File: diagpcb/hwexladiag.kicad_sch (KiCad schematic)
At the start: 0 parts

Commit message: Add HC05 symbol & footprint.
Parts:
- added J1: PINHEADER, Connector_PinHeader_2.54mm:PinHeader_1x06_P2.54mm_Vertical_SMD_Pin1Left, symbol Connector_Generic:Conn_01x06
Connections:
- new net +5V: J1.4 (Pin_4)
- new net GND: J1.6 (Pin_6)
- new net wexlaRxD: J1.3 (Pin_3)
- new net wexlaTxD: J1.2 (Pin_2)
- no-connect marks 0 -> 2
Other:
- company: (none) -> Model Railroader Club Brno I – KMŽ Brno I – https://kmz-brno.cz/
- title: (none) -> hWexla Wireless Diagnostic Adapter
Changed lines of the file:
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@@
 (kicad_sch (version 20230121) (generator eeschema)
   (paper "A5")
+  (title_block
+    (title "hWexla Wireless Diagnostic Adapter")
+    (date "2023-12-16")
+    (rev "1.0")
+    (company "Model Railroader Club Brno I – KMŽ Brno I – https://kmz-brno.cz/")
+    (comment 1 "Jan Horáček")
+    (comment 2 "https://github.com/kmzbrnoI/hwexla")
+    (comment 3 "https://creativecommons.org/licenses/by-sa/4.0/")
+    (comment 4 "Released under the Creative Commons Attribution-ShareAlike 4.0 License")
+  )
+  (no_connect (at 124.46 55.245))
+  (no_connect (at 124.46 65.405))
+  (wire (pts (xy 124.46 57.785) (xy 104.14 57.785))
+    (stroke (width 0) (type default))
+  )
+  (wire (pts (xy 111.76 62.865) (xy 124.46 62.865))
+    (stroke (width 0) (type default))
+  )
+  (wire (pts (xy 115.57 71.12) (xy 115.57 67.945))
+    (stroke (width 0) (type default))
+  )
+  (wire (pts (xy 111.76 52.07) (xy 111.76 62.865))
+    (stroke (width 0) (type default))
+  )
+  (wire (pts (xy 104.14 60.325) (xy 124.46 60.325))
+    (stroke (width 0) (type default))
+  )
+  (wire (pts (xy 115.57 67.945) (xy 124.46 67.945))
+    (stroke (width 0) (type default))
+  )
+  (label "wexlaRxD" (at 122.555 60.325 180) (fields_autoplaced)
+    (effects (font (size 1.27 1.27)) (justify right bottom))
+  )
+  (label "wexlaTxD" (at 122.555 57.785 180) (fields_autoplaced)
+    (effects (font (size 1.27 1.27)) (justify right bottom))
+  )
+  (symbol (lib_id "power:GND") (at 115.57 71.12 0) (unit 1)
+    (in_bom yes) (on_board yes) (dnp no) (fields_autoplaced)
+    (property "Reference" "#PWR01" (at 115.57 77.47 0)
+      (effects (font (size 1.27 1.27)) hide)
+    )
+    (property "Value" "GND" (at 115.57 75.2531 0)
+      (effects (font (size 1.27 1.27)))
+    )
+    (property "Footprint" "" (at 115.57 71.12 0)
+      (effects (font (size 1.27 1.27)) hide)
+    )
+    (property "Datasheet" "" (at 115.57 71.12 0)
+      (effects (font (size 1.27 1.27)) hide)
+    )
+    (pin "1")
+    (instances
+      (project "hwexladiag"
+        (path "/41af901d-6d9d-4dc3-adca-d33b9d619d2e"
+          (reference "#PWR01") (unit 1)
+        )
+      )
+    )
+  )
+  (symbol (lib_id "Connector_Generic:Conn_01x06") (at 129.54 60.325 0) (unit 1)
+    (in_bom yes) (on_board yes) (dnp no) (fields_autoplaced)
+    (property "Reference" "J1" (at 131.572 60.3829 0)
+      (effects (font (size 1.27 1.27)) (justify left))
+    )
+    (property "Value" "PINHEADER" (at 131.572 62.8071 0)
+      (effects (font (size 1.27 1.27)) (justify left))
+    )
+    (property "Footprint" "Connector_PinHeader_2.54mm:PinHeader_1x06_P2.54mm_Vertical_SMD_Pin1Left" (at 129.54 60.325 0)
+      (effects (font (size 1.27 1.27)) hide)
+    )
+    (property "Datasheet" "~" (at 129.54 60.325 0)
+      (effects (font (size 1.27 1.27)) hide)
+    )
+    (pin "1")
+    (pin "2")
+    (pin "3")
+    (pin "4")
+    (pin "5")
+    (pin "6")
+    (instances
+      (project "hwexladiag"
+        (path "/41af901d-6d9d-4dc3-adca-d33b9d619d2e"
+          (reference "J1") (unit 1)
+        )
+      )
+    )
+  )
+  (symbol (lib_id "power:+5V") (at 111.76 52.07 0) (unit 1)
+    (in_bom yes) (on_board yes) (dnp no) (fields_autoplaced)
+    (property "Reference" "#PWR02" (at 111.76 55.88 0)
+      (effects (font (size 1.27 1.27)) hide)
+    )
+    (property "Value" "+5V" (at 111.76 47.9369 0)
+      (effects (font (size 1.27 1.27)))
+    )
+    (property "Footprint" "" (at 111.76 52.07 0)
+      (effects (font (size 1.27 1.27)) hide)
+    )
+    (property "Datasheet" "" (at 111.76 52.07 0)
+      (effects (font (size 1.27 1.27)) hide)
+    )
+    (pin "1")
+    (instances
+      (project "hwexladiag"
+        (path "/41af901d-6d9d-4dc3-adca-d33b9d619d2e"
+          (reference "#PWR02") (unit 1)
+        )
+      )
+    )
+  )
   (sheet_instances
     (path "/" (page "1"))

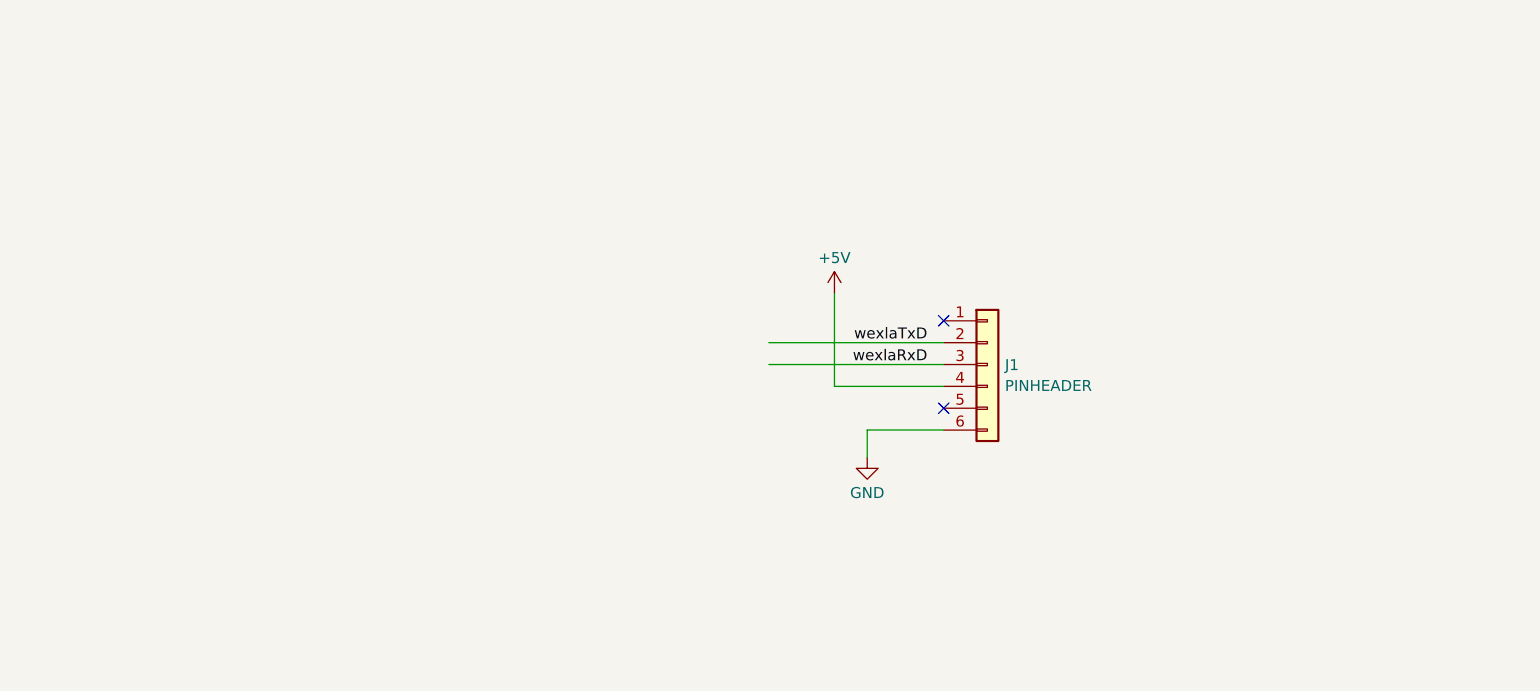
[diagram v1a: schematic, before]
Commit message: Finish diagPCB.
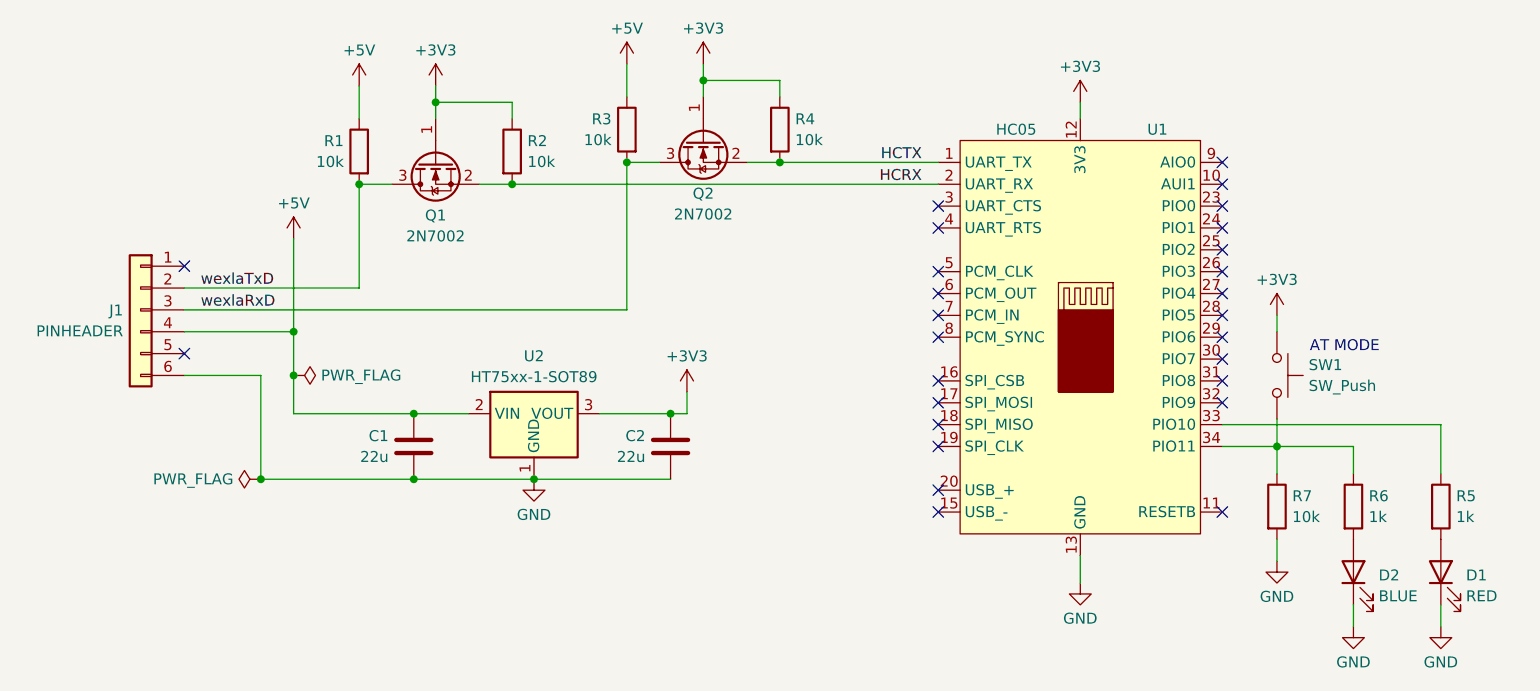
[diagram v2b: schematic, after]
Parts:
- added C1, C2: 22u, Capacitor_SMD:C_0805_2012Metric, symbol Device:C
- added D1: RED, LED_SMD:LED_0805_2012Metric, symbol Device:LED
- added D2: BLUE, LED_SMD:LED_0805_2012Metric, symbol Device:LED
- added Q1, Q2: 2N7002, Package_TO_SOT_SMD:SOT-23, symbol Transistor_FET:2N7002
- added R1, R2, R3, R4, R7: 10k, Resistor_SMD:R_0805_2012Metric, symbol Device:R
- added R5, R6: 1k, Resistor_SMD:R_0805_2012Metric, symbol Device:R
- added SW1: SW_Push, Button_Switch_SMD:SW_SPST_EVQPE1, symbol Switch:SW_Push
- added U1: HC05, hc05:HC05, symbol hc05:HC05
- added U2: HT75xx-1-SOT89, Package_TO_SOT_SMD:SOT-89-3, symbol Regulator_Linear:HT75xx-1-SOT89
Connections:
- net +5V: now also C1.1, R1.1, R3.1, U2.2 (VIN)
- net GND: now also C1.2, C2.2, D1.1 (K), D2.1 (K), R7.2, U1.13 (GND), U1.21 (GND), U1.22 (GND), U2.1 (GND)
- net wexlaRxD: now also Q2.3 (D), R3.2
- net wexlaTxD: now also Q1.3 (D), R1.2
- new net: D1.2 (A), R5.2
- new net: D2.2 (A), R6.2
- new net: R6.1, R7.1, SW1.2, U1.34 (PIO11)
- new net: R5.1, U1.33 (PIO10)
- new net +3V3: C2.1, Q1.1 (G), Q2.1 (G), R2.1, R4.1, SW1.1, U1.12 (3V3), U2.3 (VOUT)
- new net HCRX: Q1.2 (S), R2.2, U1.2 (UART_RX)
- new net HCTX: Q2.2 (S), R4.2, U1.1 (UART_TX)
- no-connect marks 2 -> 27
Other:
- note added: "AT MODE"
- moved on the sheet: J1

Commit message: diag: remove blue LED.
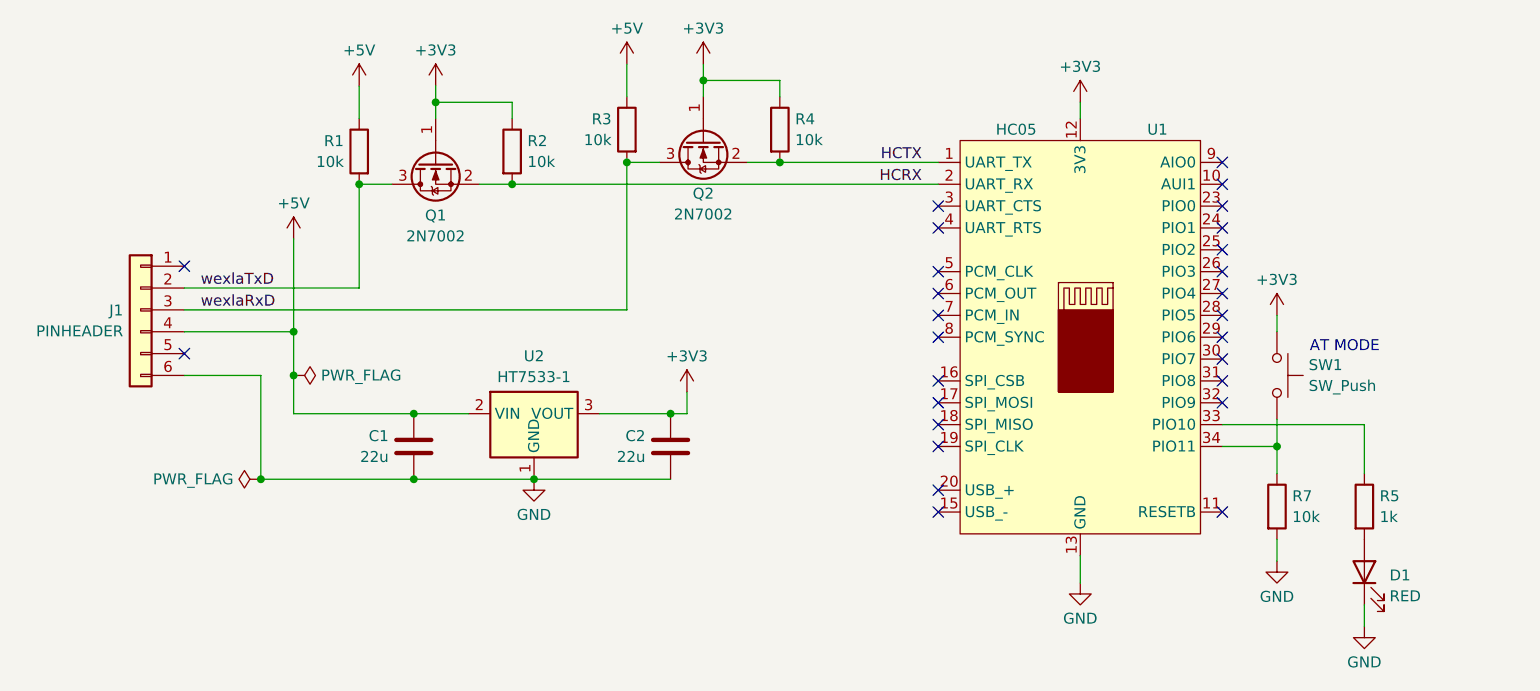
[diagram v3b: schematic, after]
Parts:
- removed D2: BLUE, LED_SMD:LED_0805_2012Metric, symbol Device:LED
- removed R6: 1k, Resistor_SMD:R_0805_2012Metric, symbol Device:R
- U2: value HT75xx-1-SOT89 -> HT7533-1
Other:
- moved on the sheet: D1, R5
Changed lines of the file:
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@@
   (title_block
     (title "hWexla Wireless Diagnostic Adapter")
-    (date "2023-12-16")
-    (rev "1.0")
+    (date "2024-02-27")
+    (rev "1.1")
     (company "Model Railroader Club Brno I – KMŽ Brno I – https://kmz-brno.cz/")
     (comment 1 "Jan Horáček")
@@
     (stroke (width 0) (type default))
   )
-  (wire (pts (xy 172.085 88.265) (xy 172.085 90.805))
-    (stroke (width 0) (type default))
-  )
   (wire (pts (xy 48.895 61.595) (xy 48.895 56.515))
     (stroke (width 0) (type default))
   )
-  (wire (pts (xy 182.245 67.31) (xy 182.245 73.025))
+  (wire (pts (xy 173.355 67.31) (xy 173.355 73.025))
     (stroke (width 0) (type default))
   )
@@
     (stroke (width 0) (type default))
   )
-  (wire (pts (xy 163.195 69.85) (xy 172.085 69.85))
-    (stroke (width 0) (type default))
-  )
   (wire (pts (xy 62.865 66.04) (xy 69.215 66.04))
     (stroke (width 0) (type default))
@@
     (stroke (width 0) (type default))
   )
-  (wire (pts (xy 172.085 69.85) (xy 172.085 73.025))
-    (stroke (width 0) (type default))
-  )
   (wire (pts (xy 163.195 69.85) (xy 163.195 66.675))
     (stroke (width 0) (type default))
   )
-  (wire (pts (xy 156.845 67.31) (xy 182.245 67.31))
+  (wire (pts (xy 156.845 67.31) (xy 173.355 67.31))
     (stroke (width 0) (type default))
   )
@@
     (stroke (width 0) (type default))
   )
-  (wire (pts (xy 182.245 88.265) (xy 182.245 90.805))
+  (wire (pts (xy 173.355 88.265) (xy 173.355 90.805))
     (stroke (width 0) (type default))
   )
@@
     )
   )
-  (symbol (lib_id "Device:LED") (at 182.245 84.455 90) (unit 1)
-    (in_bom yes) (on_board yes) (dnp no) (fields_autoplaced)
-    (property "Reference" "D1" (at 185.166 84.8304 90)
+  (symbol (lib_id "Device:LED") (at 173.355 84.455 90) (unit 1)
+    (in_bom yes) (on_board yes) (dnp no) (fields_autoplaced)
+    (property "Reference" "D1" (at 176.276 84.8304 90)
       (effects (font (size 1.27 1.27)) (justify right))
     )
-    (property "Value" "RED" (at 185.166 87.2546 90)
+    (property "Value" "RED" (at 176.276 87.2546 90)
       (effects (font (size 1.27 1.27)) (justify right))
     )
-    (property "Footprint" "LED_SMD:LED_0805_2012Metric" (at 182.245 84.455 0)
-      (effects (font (size 1.27 1.27)) hide)
-    )
-    (property "Datasheet" "~" (at 182.245 84.455 0)
+    (property "Footprint" "LED_SMD:LED_0805_2012Metric" (at 173.355 84.455 0)
+      (effects (font (size 1.27 1.27)) hide)
+    )
+    (property "Datasheet" "~" (at 173.355 84.455 0)
       (effects (font (size 1.27 1.27)) hide)
     )
@@
     )
   )
-  (symbol (lib_id "Device:LED") (at 172.085 84.455 90) (unit 1)
-    (in_bom yes) (on_board yes) (dnp no) (fields_autoplaced)
-    (property "Reference" "D2" (at 175.006 84.8304 90)
-      (effects (font (size 1.27 1.27)) (justify right))
-    )
-    (property "Value" "BLUE" (at 175.006 87.2546 90)
-      (effects (font (size 1.27 1.27)) (justify right))
-    )
-    (property "Footprint" "LED_SMD:LED_0805_2012Metric" (at 172.085 84.455 0)
-      (effects (font (size 1.27 1.27)) hide)
-    )
-    (property "Datasheet" "~" (at 172.085 84.455 0)
-      (effects (font (size 1.27 1.27)) hide)
-    )
-    (pin "1")
-    (pin "2")
-    (instances
-      (project "hwexladiag"
-        (path "/41af901d-6d9d-4dc3-adca-d33b9d619d2e"
-          (reference "D2") (unit 1)
-        )
-      )
-    )
-  )
   (symbol (lib_id "Transistor_FET:2N7002") (at 65.405 36.83 90) (mirror x) (unit 1)
     (in_bom yes) (on_board yes) (dnp no)
@@
     )
   )
-  (symbol (lib_id "power:GND") (at 182.245 90.805 0) (unit 1)
-    (in_bom yes) (on_board yes) (dnp no) (fields_autoplaced)
-    (property "Reference" "#PWR011" (at 182.245 97.155 0)
-      (effects (font (size 1.27 1.27)) hide)
-    )
-    (property "Value" "GND" (at 182.245 94.9381 0)
-      (effects (font (size 1.27 1.27)))
-    )
-    (property "Footprint" "" (at 182.245 90.805 0)
-      (effects (font (size 1.27 1.27)) hide)
-    )
-    (property "Datasheet" "" (at 182.245 90.805 0)
+  (symbol (lib_id "power:GND") (at 173.355 90.805 0) (unit 1)
+    (in_bom yes) (on_board yes) (dnp no) (fields_autoplaced)
+    (property "Reference" "#PWR011" (at 173.355 97.155 0)
+      (effects (font (size 1.27 1.27)) hide)
+    )
+    (property "Value" "GND" (at 173.355 94.9381 0)
+      (effects (font (size 1.27 1.27)))
+    )
+    (property "Footprint" "" (at 173.355 90.805 0)
+      (effects (font (size 1.27 1.27)) hide)
+    )
+    (property "Datasheet" "" (at 173.355 90.805 0)
       (effects (font (size 1.27 1.27)) hide)
     )
@@
       (effects (font (size 1.27 1.27)))
     )
-    (property "Value" "HT75xx-1-SOT89" (at 76.835 61.7799 0)
+    (property "Value" "HT7533-1" (at 76.835 61.7799 0)
       (effects (font (size 1.27 1.27)))
     )
@@
     )
   )
-  (symbol (lib_id "Device:R") (at 182.245 76.835 0) (unit 1)
-    (in_bom yes) (on_board yes) (dnp no) (fields_autoplaced)
-    (property "Reference" "R5" (at 184.023 75.6229 0)
-      (effects (font (size 1.27 1.27)) (justify left))
-    )
-    (property "Value" "1k" (at 184.023 78.0471 0)
-      (effects (font (size 1.27 1.27)) (justify left))
-    )
-    (property "Footprint" "Resistor_SMD:R_0805_2012Metric" (at 180.467 76.835 90)
-      (effects (font (size 1.27 1.27)) hide)
-    )
-    (property "Datasheet" "~" (at 182.245 76.835 0)
+  (symbol (lib_id "Device:R") (at 173.355 76.835 0) (unit 1)
+    (in_bom yes) (on_board yes) (dnp no) (fields_autoplaced)
+    (property "Reference" "R5" (at 175.133 75.6229 0)
+      (effects (font (size 1.27 1.27)) (justify left))
+    )
+    (property "Value" "1k" (at 175.133 78.0471 0)
+      (effects (font (size 1.27 1.27)) (justify left))
+    )
+    (property "Footprint" "Resistor_SMD:R_0805_2012Metric" (at 171.577 76.835 90)
+      (effects (font (size 1.27 1.27)) hide)
+    )
+    (property "Datasheet" "~" (at 173.355 76.835 0)
       (effects (font (size 1.27 1.27)) hide)
     )
@@
     )
   )
-  (symbol (lib_id "Device:R") (at 172.085 76.835 0) (unit 1)
-    (in_bom yes) (on_board yes) (dnp no) (fields_autoplaced)
-    (property "Reference" "R6" (at 173.863 75.6229 0)
-      (effects (font (size 1.27 1.27)) (justify left))
-    )
-    (property "Value" "1k" (at 173.863 78.0471 0)
-      (effects (font (size 1.27 1.27)) (justify left))
-    )
-    (property "Footprint" "Resistor_SMD:R_0805_2012Metric" (at 170.307 76.835 90)
-      (effects (font (size 1.27 1.27)) hide)
-    )
-    (property "Datasheet" "~" (at 172.085 76.835 0)
-      (effects (font (size 1.27 1.27)) hide)
-    )
-    (pin "1")
-    (pin "2")
-    (instances
-      (project "hwexladiag"
-        (path "/41af901d-6d9d-4dc3-adca-d33b9d619d2e"
-          (reference "R6") (unit 1)
-        )
-      )
-    )
-  )
   (symbol (lib_id "power:GND") (at 140.335 85.725 0) (mirror y) (unit 1)
     (in_bom yes) (on_board yes) (dnp no) (fields_autoplaced)
@@
         )
       )
-    )
-  )
-  (symbol (lib_id "power:GND") (at 172.085 90.805 0) (unit 1)
-    (in_bom yes) (on_board yes) (dnp no) (fields_autoplaced)
-    (property "Reference" "#PWR012" (at 172.085 97.155 0)
-      (effects (font (size 1.27 1.27)) hide)
-    )
-    (property "Value" "GND" (at 172.085 94.9381 0)
-      (effects (font (size 1.27 1.27)))
-    )
-    (property "Footprint" "" (at 172.085 90.805 0)
-      (effects (font (size 1.27 1.27)) hide)
-    )
-    (property "Datasheet" "" (at 172.085 90.805 0)
-      (effects (font (size 1.27 1.27)) hide)
-    )
-    (pin "1")
-    (instances
-      (project "hwexladiag"
-        (path "/41af901d-6d9d-4dc3-adca-d33b9d619d2e"
-          (reference "#PWR012") (unit 1)
-        )
-      )
